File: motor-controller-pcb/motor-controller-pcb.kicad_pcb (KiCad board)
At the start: 2 copper layers, 90 x 65 mm, 15 parts, among them J1 Conn_01x06_Pin, J2 Conn_01x06_Pin, J3 Conn_01x06_Pin, J4 Conn_01x06_Pin, J5 Conn_01x04_Pin, J6 Conn_01x04_Pin, M1 Conn_01x02_Pin, M2 Conn_01x02_Pin, M3 Conn_01x02_Pin, M4 Conn_01x02_Pin

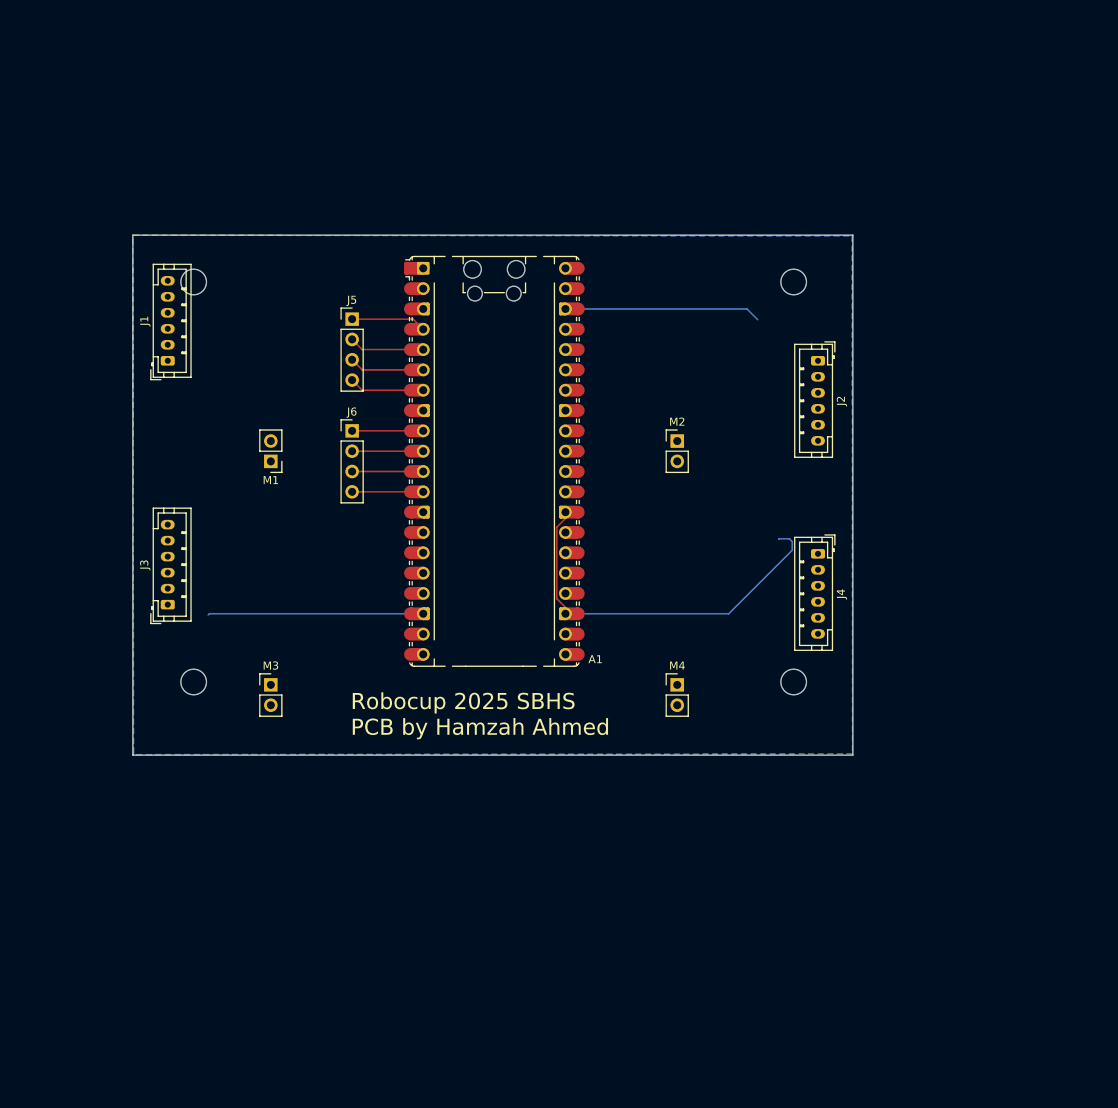
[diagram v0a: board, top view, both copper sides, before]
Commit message: feat: pcb layout
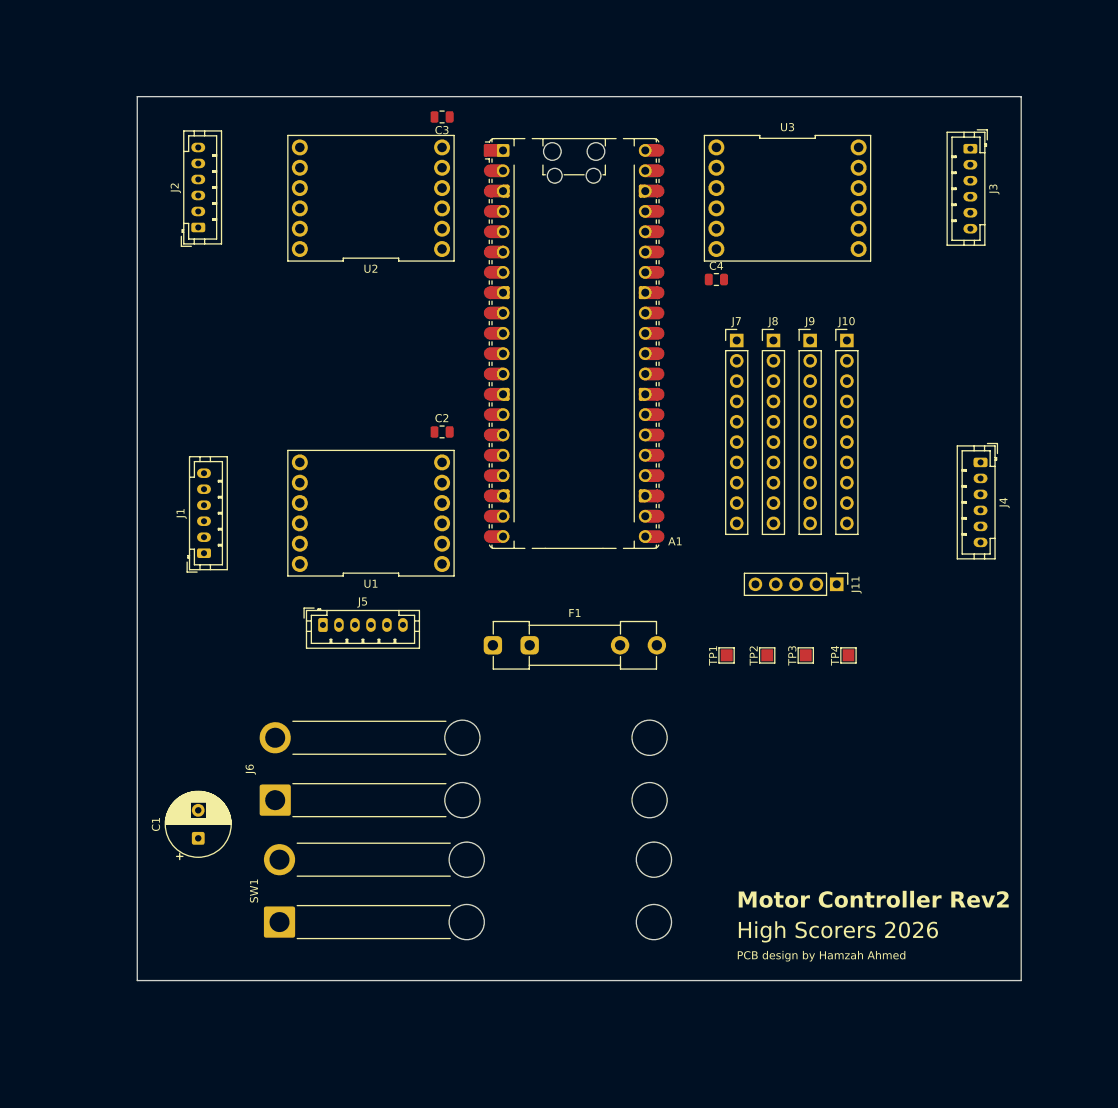
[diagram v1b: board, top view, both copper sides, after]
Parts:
- removed M1, M2, M3, M4: Conn_01x02_Pin, Connector_PinHeader_2.54mm:PinHeader_1x02_P2.54mm_Vertical
- removed REF** (x4): MountingHole_3.2mm_M3, MountingHole:MountingHole_3.2mm_M3
- added C1: 470uF, Capacitor_THT:CP_Radial_D8.0mm_P3.50mm, F.Cu at (115.6, 129.5)
- added C2: 100nF, Capacitor_SMD:C_0805_2012Metric, F.Cu at (146.1, 78.7)
- added C3: 100nF, Capacitor_SMD:C_0805_2012Metric, F.Cu at (146.1, 39.4)
- added C4: 100nF, Capacitor_SMD:C_0805_2012Metric, F.Cu at (180.3, 59.7)
- added F1: Fuse, Fuse:Fuseholder_Clip-5x20mm_Littelfuse_100_Inline_P20.50x4.60mm_D1.30mm_Horizontal, F.Cu at (152.4, 105.4)
- added J10: 3V3, Connector_PinHeader_2.54mm:PinHeader_1x10_P2.54mm_Vertical, F.Cu at (196.7, 67.3)
- added J11: Conn_01x05_Pin, Connector_PinHeader_2.54mm:PinHeader_1x05_P2.54mm_Vertical, F.Cu at (195.4, 97.8)
- added J7: GND, Connector_PinHeader_2.54mm:PinHeader_1x10_P2.54mm_Vertical, F.Cu at (182.9, 67.3)
- added J8: 5V, Connector_PinHeader_2.54mm:PinHeader_1x10_P2.54mm_Vertical, F.Cu at (187.5, 67.3)
- added J9: V_Batt, Connector_PinHeader_2.54mm:PinHeader_1x10_P2.54mm_Vertical, F.Cu at (192.1, 67.3)
- added SW1: Battery Switch, Connector_Wire:SolderWire-2sqmm_1x02_P7.8mm_D2mm_OD3.9mm_Relief2x, F.Cu at (125.7, 140.0)
- added TP1: 5V TestPoint, TestPoint:TestPoint_Pad_1.5x1.5mm, F.Cu at (181.6, 106.7)
- added TP2: GND TestPoint, TestPoint:TestPoint_Pad_1.5x1.5mm, F.Cu at (186.7, 106.7)
- added TP3: V_Batt Test Point, TestPoint:TestPoint_Pad_1.5x1.5mm, F.Cu at (191.5, 106.7)
- added TP4: 3V3 Test Point, TestPoint:TestPoint_Pad_1.5x1.5mm, F.Cu at (196.8, 106.7)
- added U1: ~, robocup-library:DRI044, F.Cu at (137.2, 88.9)
- added U2: ~, robocup-library:DRI044, F.Cu at (137.2, 49.5)
- added U3: ~, robocup-library:DRI044, F.Cu at (189.2, 49.5)
- J1: value Conn_01x06_Pin -> Motor 1
- J2: value Conn_01x06_Pin -> Motor 2
- J3: value Conn_01x06_Pin -> Motor 3
- J4: value Conn_01x06_Pin -> Motor 4
- J5: value Conn_01x04_Pin -> Dribbler Motor; footprint Connector_PinHeader_2.54mm:PinHeader_1x04_P2.54mm_Vertical -> Connector_JST:JST_PH_B6B-PH-K_1x06_P2.00mm_Vertical
- J6: value Conn_01x04_Pin -> Battery Connector; footprint Connector_PinHeader_2.54mm:PinHeader_1x04_P2.54mm_Vertical -> Connector_Wire:SolderWire-2sqmm_1x02_P7.8mm_D2mm_OD3.9mm_Relief2x
- moved J3 115.4 mm to (212.1, 43.3), turned to -90 degrees
- moved J2 79.2 mm to (115.6, 53.2), turned to 90 degrees
- moved J6 47.2 mm to (125.2, 124.8), turned to 90 degrees
- moved J5 38.4 mm to (131.2, 102.9)
- moved J1 24.5 mm to (116.3, 93.9)
- moved J4 23.3 mm to (213.4, 82.5)
- moved A1 17.8 mm to (162.6, 67.7)
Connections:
- A1 pad 1: unconnected-(A1-GPIO0-Pad1) -> /DIR_DRIB
- A1 pad 10: Net-(A1-GPIO7) -> /PWM3
- A1 pad 11: Net-(A1-GPIO8) -> /PWM4
- A1 pad 12: Net-(A1-GPIO9) -> /DIR4
- A1 pad 14: unconnected-(A1-GPIO10-Pad14)_1 -> /GPIO10
- A1 pad 2: unconnected-(A1-GPIO1-Pad2)_1 -> /PWM_DRIB
- A1 pad 20: unconnected-(A1-GPIO15-Pad20) -> /GPIO15
- A1 pad 21: unconnected-(A1-GPIO16-Pad21)_1 -> /GPIO16
- A1 pad 22: unconnected-(A1-GPIO17-Pad22) -> /GPIO17
- A1 pad 24: unconnected-(A1-GPIO18-Pad24)_1 -> /GPIO18
- A1 pad 36: unconnected-(A1-3V3-Pad36)_1 -> +3V3
- A1 pad 4: Net-(A1-GPIO2) -> /DIR1
- A1 pad 5: Net-(A1-GPIO3) -> /PWM1
- A1 pad 6: Net-(A1-GPIO4) -> /PWM2
- A1 pad 7: Net-(A1-GPIO5) -> /DIR2
- A1 pad 9: Net-(A1-GPIO6) -> /DIR3
- J5 pad 1: Net-(A1-GPIO2) -> Net-(J5-Pin_1)
- J5 pad 2: Net-(A1-GPIO3) -> unconnected-(J5-Pin_2-Pad2)
- J5 pad 3: Net-(A1-GPIO4) -> unconnected-(J5-Pin_3-Pad3)
- J5 pad 4: Net-(A1-GPIO5) -> unconnected-(J5-Pin_4-Pad4)
- J6 pad 1: Net-(A1-GPIO6) -> Net-(J6-Pin_1)
- J6 pad 2: Net-(A1-GPIO7) -> GND
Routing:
- net GND: track 100.4 -> 0.00 mm
- net Net-(A1-GPIO2): track 9.42 -> 0.00 mm
- net Net-(A1-GPIO9): track 8.89 -> 0.00 mm
- net Net-(A1-GPIO6): track 8.89 -> 0.00 mm
- net Net-(A1-GPIO5): track 8.62 -> 0.00 mm
- net Net-(A1-GPIO4): track 8.62 -> 0.00 mm
- net Net-(A1-GPIO3): track 8.62 -> 0.00 mm
- net Net-(A1-GPIO8): track 8.09 -> 0.00 mm
- net Net-(A1-GPIO7): track 8.09 -> 0.00 mm
- net /Encoder 2A: track 1.22 -> 0.00 mm
- net /Encoder 1B: track 1.13 -> 0.00 mm
- removed copper zone on B.Cu, net GND
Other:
- board size 90 x 65 mm -> 110.5 x 110.5 mm
- board text added: "High Scorers 2026"
- board text added: "Motor Controller Rev2"
- board text added: "PCB design by Hamzah Ahmed"
- board text removed: "Robocup 2025 SBHS PCB by Hamzah Ahmed"

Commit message: feat: final
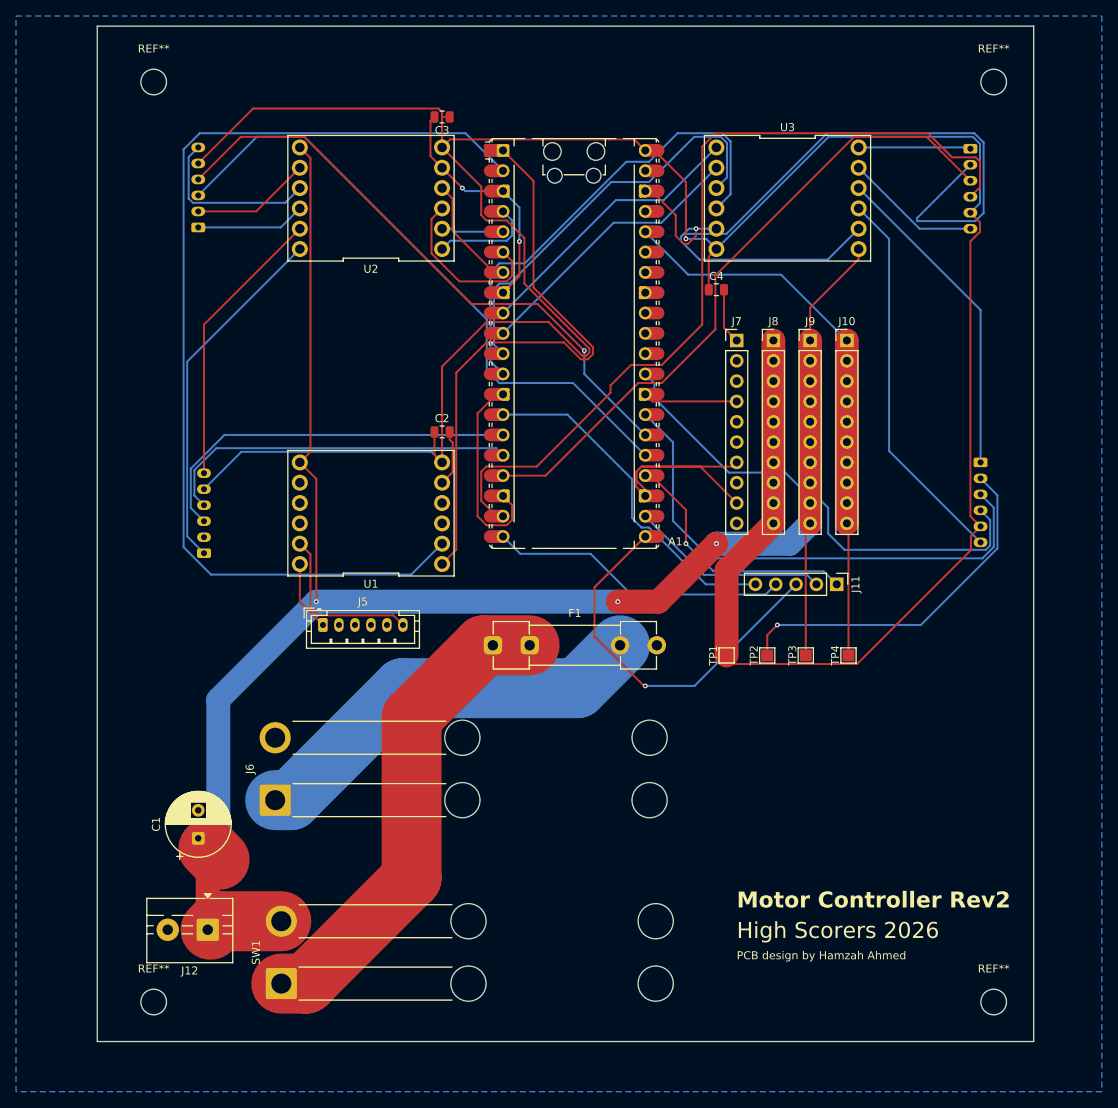
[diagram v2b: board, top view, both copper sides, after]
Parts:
- added J12: V_Batt, TerminalBlock:TerminalBlock_MaiXu_MX126-5.0-02P_1x02_P5.00mm, F.Cu at (116.8, 141.0)
- added REF**: MountingHole_3.2mm_M3, MountingHole:MountingHole_3.2mm_M3, F.Cu at (215.0, 150.0)
- added REF**: MountingHole_3.2mm_M3, MountingHole:MountingHole_3.2mm_M3, F.Cu at (110.0, 150.0)
- added REF**: MountingHole_3.2mm_M3, MountingHole:MountingHole_3.2mm_M3, F.Cu at (215.0, 35.0)
- added REF**: MountingHole_3.2mm_M3, MountingHole:MountingHole_3.2mm_M3, F.Cu at (110.0, 35.0)
- J1, J2, J3, J4: moved to B.Cu
- moved SW1 7.69 mm to (126.0, 147.7)
- moved C4 1.27 mm to (180.3, 61.0)
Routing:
- net +5V: track 0.00 -> 365.8 mm, vias 0 -> 1
- net GND: track 0.00 -> 290.3 mm, vias 0 -> 4
- net +BATT: track 0.00 -> 235.1 mm, vias 0 -> 3
- net /PWM_DRIB: track 0.00 -> 127.8 mm
- net /Encoder 3B: track 0.00 -> 106.2 mm
- net /Encoder 3A: track 0.00 -> 82.2 mm
- net /Encoder 2A: track 0.00 -> 79.1 mm
- net /Encoder 2B: track 0.00 -> 75.2 mm, vias 0 -> 1
- net /DIR_DRIB: track 0.00 -> 74.6 mm
- net +3V3: track 0.00 -> 70.3 mm
- net /Encoder 4A: track 0.00 -> 64.6 mm
- net Net-(SW1-A): track 0.00 -> 60.3 mm
- net /Encoder 4B: track 0.00 -> 60.3 mm
- net /DIR4: track 0.00 -> 60.1 mm
- net /PWM4: track 0.00 -> 52.1 mm
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- added copper zone on B.Cu, net GND
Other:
- board size 110.5 x 110.5 mm -> 117 x 126.9 mm
